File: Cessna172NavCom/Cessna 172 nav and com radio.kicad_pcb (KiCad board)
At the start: 2 copper layers, 180 x 98 mm, 95 parts, among them J1 EN11-HSM1BF20, J2 USB_B_Micro, J3 EN11-HSM1BF20, J4 EN11-HSM1BF20, J5 EN11-HSM1BF20, J6 EN11-HSM1BF20, J7 EN11-HSM1BF20, J8 Conn_02x20_Odd_Even, SW1 SW_Push, SW2 SW_Push, SW3 SW_Push, SW4 SW_Push, SW5 SW_Push, SW6 SW_Push, U1 MAX7219 COM standby, U10 3651A, U11 MAX7219 COM standby, U12 3651A, U13 MAX7219 COM standby, U14 3651A, U15 MAX7219 COM standby, U16 3651A, U2 3651A, U3 MAX7219 COM standby, U4 3651A, U5 MAX7219 COM standby, U6 3651A, U7 MAX7219 COM standby, U8 3651A, U9 MAX7219 COM standby

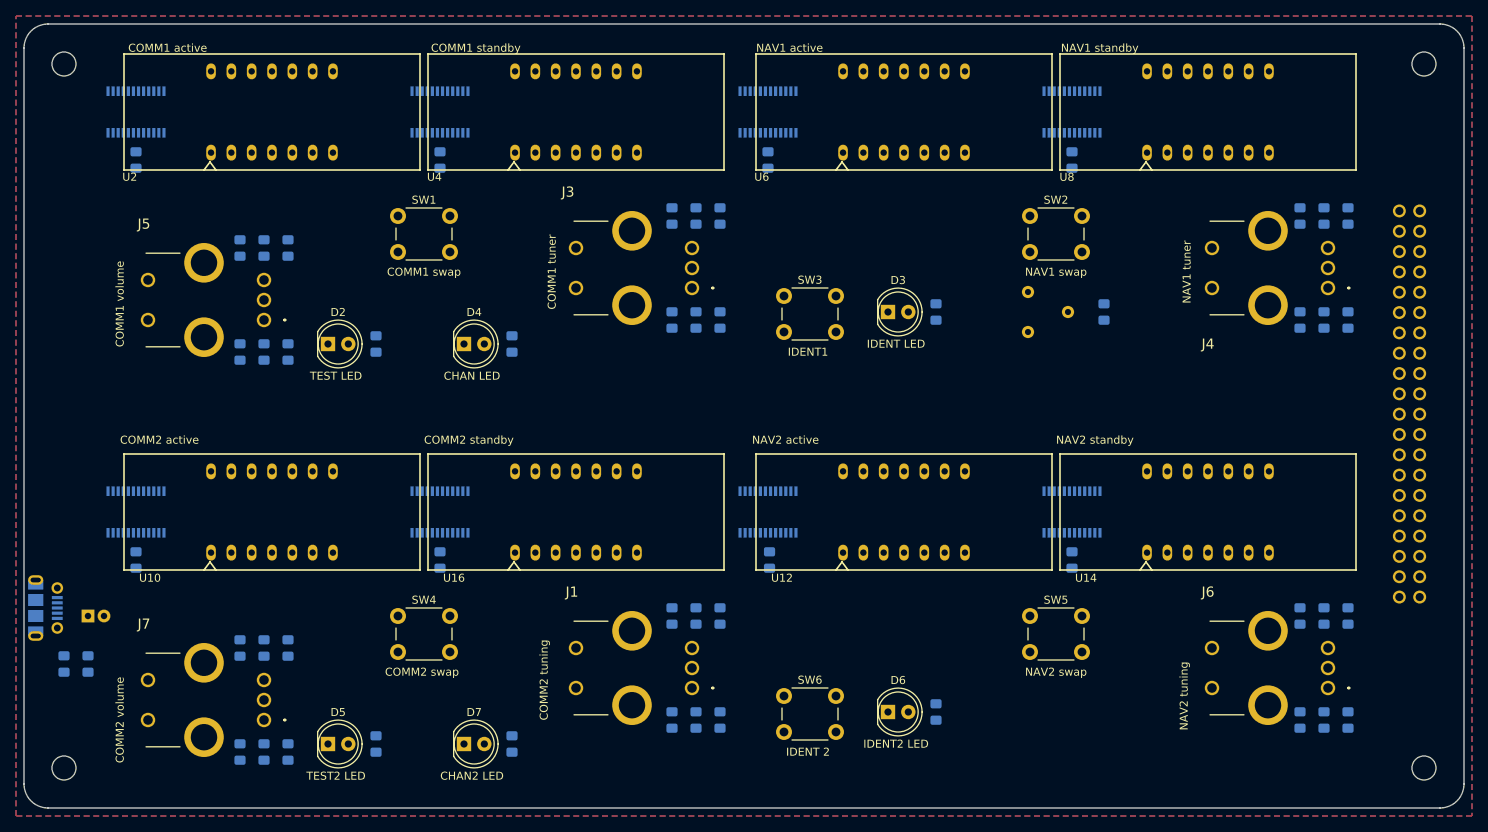
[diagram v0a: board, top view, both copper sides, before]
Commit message: Fully routed woot woot!
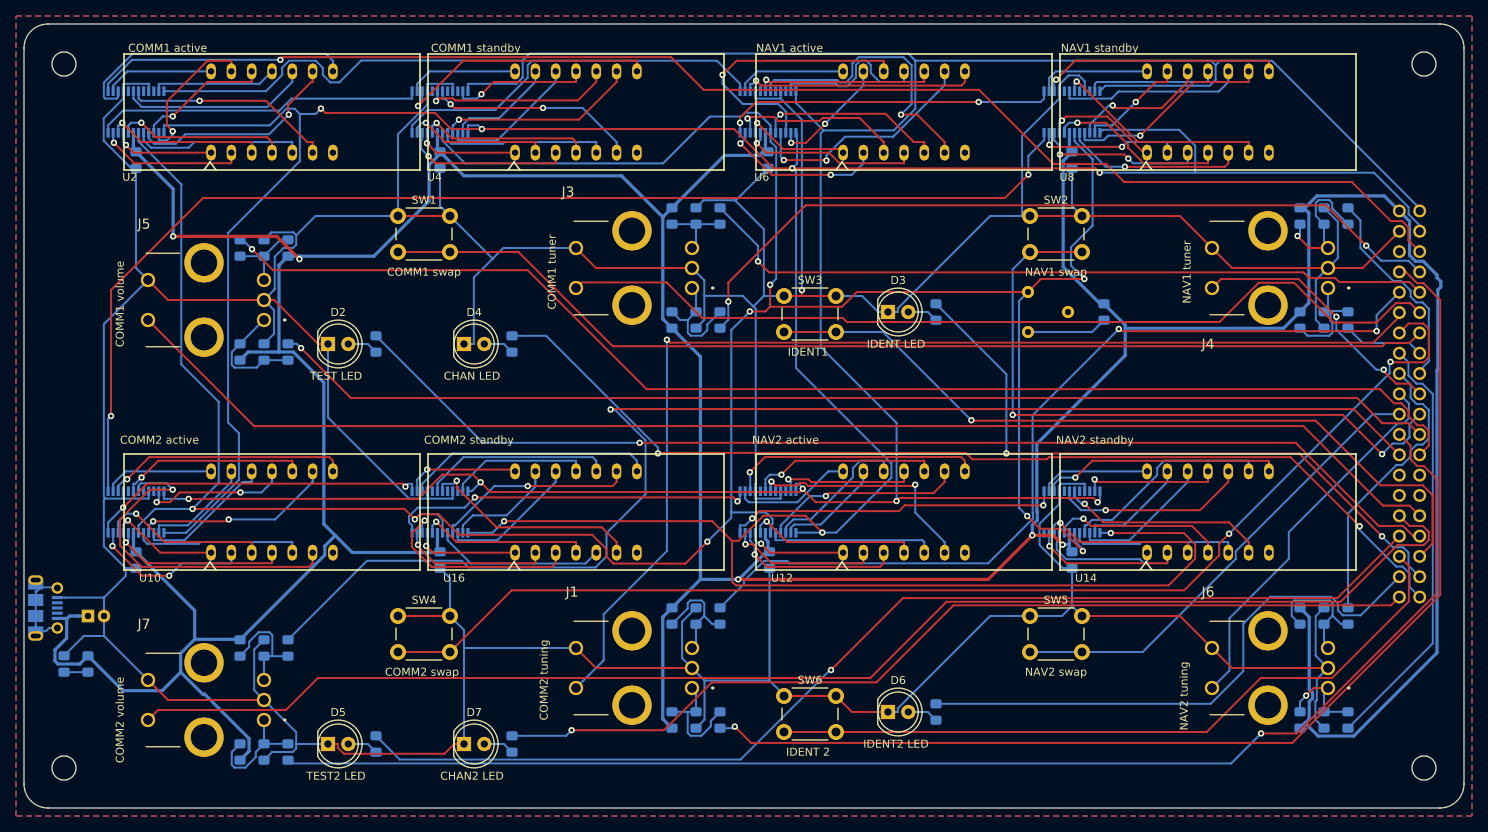
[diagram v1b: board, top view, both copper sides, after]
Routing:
- net GND: track 0.00 -> 799.6 mm, vias 0 -> 1
- net +5V: track 0.00 -> 595.3 mm, vias 0 -> 5
- net CLK: track 0.00 -> 438.1 mm, vias 0 -> 7
- net LOAD: track 0.00 -> 400.2 mm, vias 0 -> 5
- net ISET: track 0.00 -> 349.0 mm, vias 0 -> 8
- net DIN: track 0.00 -> 177.3 mm, vias 0 -> 1
- net TEST2_SW: track 0.00 -> 174.9 mm
- net COMM2_VOL_LEFT: track 0.00 -> 174.8 mm, vias 0 -> 1
- net TEST1_SW: track 0.00 -> 169.1 mm
- net COMM2_VOL_RIGHT: track 0.00 -> 168.3 mm, vias 0 -> 1
- net COMM1_VOL_RIGHT: track 0.00 -> 162.4 mm, vias 0 -> 1
- net COMM2_TX_SW: track 0.00 -> 153.8 mm, vias 0 -> 2
- net /sheet5F68A9C2/DIN: track 0.00 -> 152.0 mm, vias 0 -> 2
- net COMM1_VOL_LEFT: track 0.00 -> 146.2 mm, vias 0 -> 1
- net COMM2_LEFT: track 0.00 -> 142.1 mm, vias 0 -> 1
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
